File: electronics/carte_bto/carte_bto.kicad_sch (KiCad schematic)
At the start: 59 parts, among them J1 DIN41612_02x32_AB, J2 Conn_01x01, J3 Conn_01x01, J4 Conn_01x01, Q17 MMBT2222A, Q19 MMBT2222A, U1 LTC1859IG_PBF, U2 74AHC541, U3 74AHC541, U4 LT6654AIS6-2.5_TRPBF

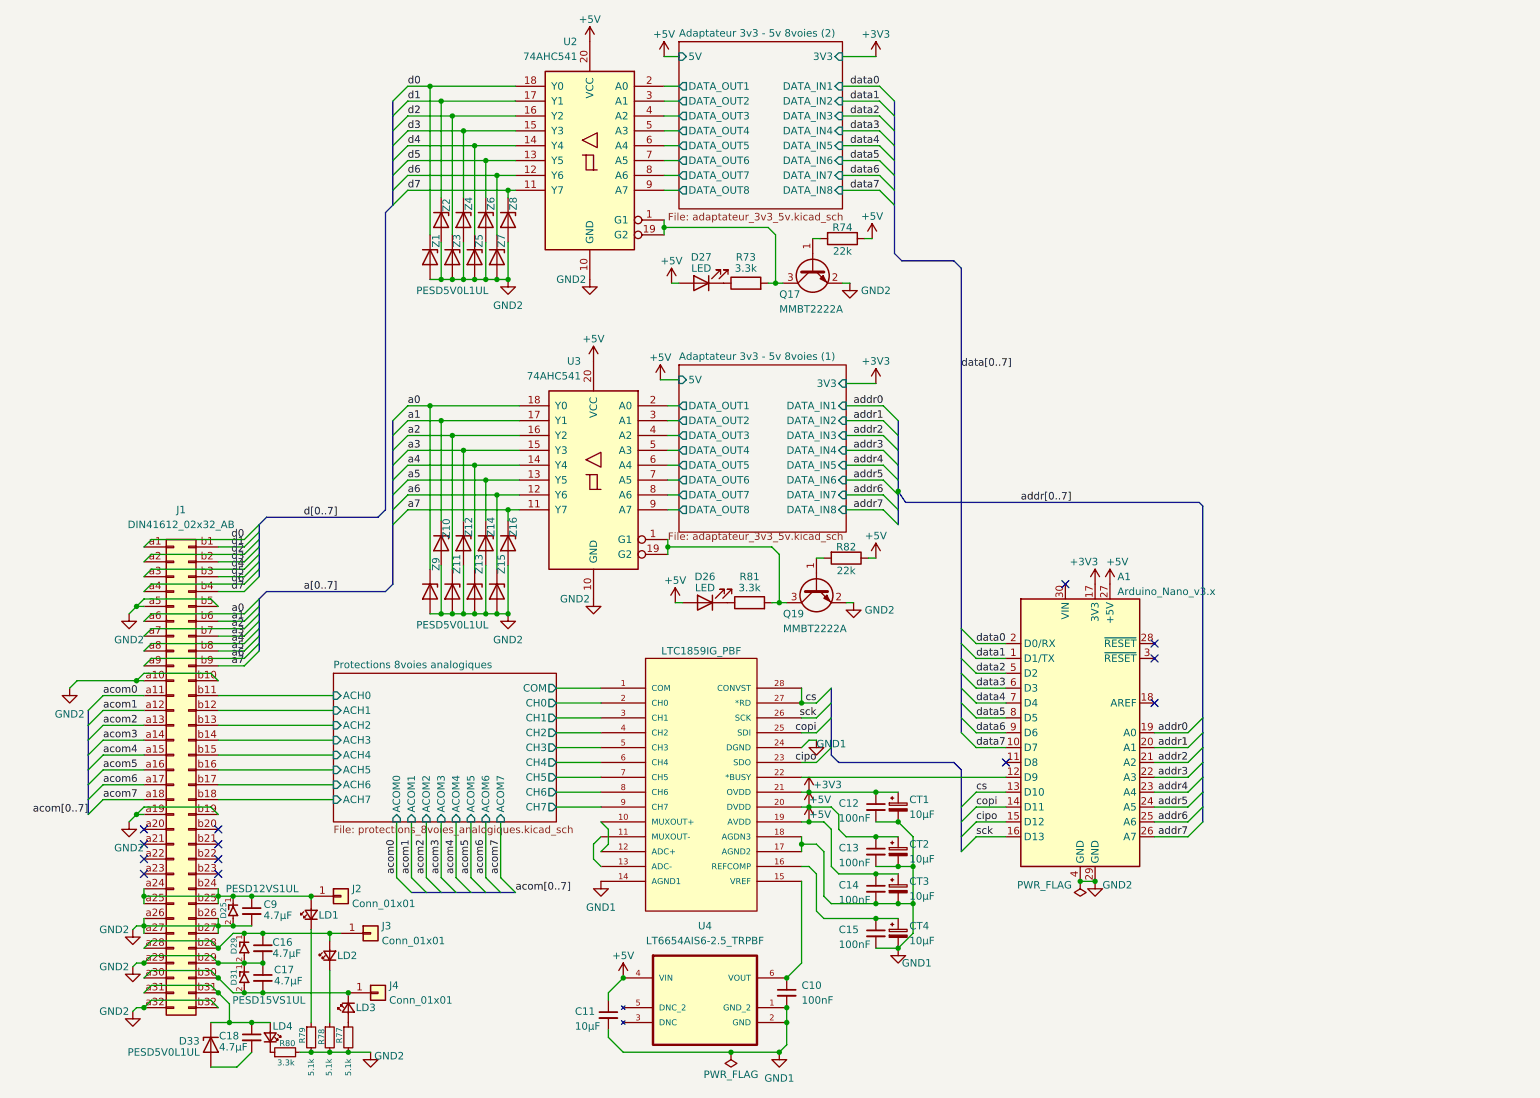
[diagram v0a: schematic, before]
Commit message: BTO schematic: cleanup and documentation
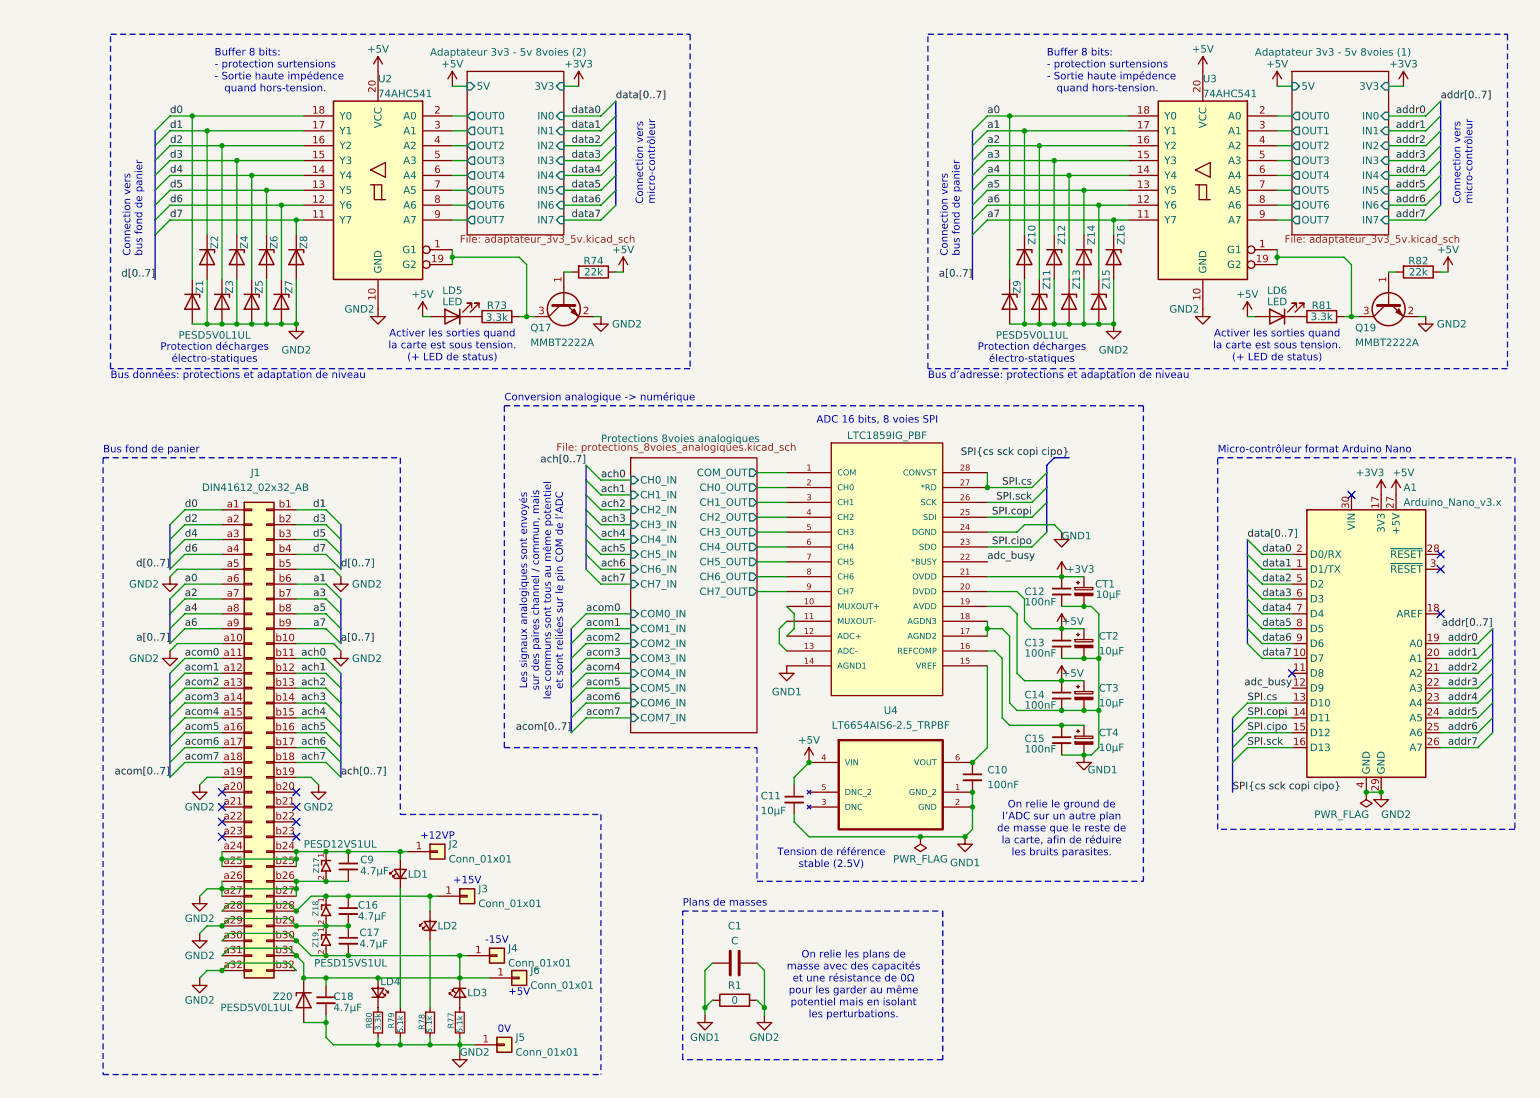
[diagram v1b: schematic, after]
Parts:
- added C1: C, symbol Device:C
- added J5, J6: Conn_01x01, symbol Connector_Generic:Conn_01x01
- added R1: 0, symbol Device:R
- renumbered D27 to LD5, D26 to LD6, D25 to Z17, D29 to Z18, D31 to Z19, D33 to Z20
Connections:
- net GND1: now also C1.1, R1.1
- net GND2: now also C18.2, R80.1, Z20.2 (A), C1.2, J5.1 (Pin_1), R1.2; no longer R80.2
- net at C18.1, J1.a31 (Pin_a31), J1.b31 (Pin_b31)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: now also C17.2, J1.a30 (Pin_a30), J1.b30 (Pin_b30), J4.1 (Pin_1), LD3.1 (K), Z19.2, J6.1 (Pin_1)
- net adc_busy: now reaches A1.12 (D9), U1.22 (*BUSY)
- net at LD4.1 (K): now also R80.2; no longer R80.1
- net Adaptateur 3v3 - 5v 8voies (1)/DATA_OUT1 renamed Adaptateur 3v3 - 5v 8voies (1)/OUT0
- net Adaptateur 3v3 - 5v 8voies (1)/DATA_OUT2 renamed Adaptateur 3v3 - 5v 8voies (1)/OUT1
- net Adaptateur 3v3 - 5v 8voies (1)/DATA_OUT3 renamed Adaptateur 3v3 - 5v 8voies (1)/OUT2
- net Adaptateur 3v3 - 5v 8voies (1)/DATA_OUT4 renamed Adaptateur 3v3 - 5v 8voies (1)/OUT3
- net Adaptateur 3v3 - 5v 8voies (1)/DATA_OUT5 renamed Adaptateur 3v3 - 5v 8voies (1)/OUT4
- net Adaptateur 3v3 - 5v 8voies (1)/DATA_OUT6 renamed Adaptateur 3v3 - 5v 8voies (1)/OUT5
- net Adaptateur 3v3 - 5v 8voies (1)/DATA_OUT7 renamed Adaptateur 3v3 - 5v 8voies (1)/OUT6
- net Adaptateur 3v3 - 5v 8voies (1)/DATA_OUT8 renamed Adaptateur 3v3 - 5v 8voies (1)/OUT7
- net Adaptateur 3v3 - 5v 8voies (2)/DATA_OUT1 renamed Adaptateur 3v3 - 5v 8voies (2)/OUT0
- net Adaptateur 3v3 - 5v 8voies (2)/DATA_OUT2 renamed Adaptateur 3v3 - 5v 8voies (2)/OUT1
- net Adaptateur 3v3 - 5v 8voies (2)/DATA_OUT3 renamed Adaptateur 3v3 - 5v 8voies (2)/OUT2
- net Adaptateur 3v3 - 5v 8voies (2)/DATA_OUT4 renamed Adaptateur 3v3 - 5v 8voies (2)/OUT3
- net Adaptateur 3v3 - 5v 8voies (2)/DATA_OUT5 renamed Adaptateur 3v3 - 5v 8voies (2)/OUT4
- net Adaptateur 3v3 - 5v 8voies (2)/DATA_OUT6 renamed Adaptateur 3v3 - 5v 8voies (2)/OUT5
- net Adaptateur 3v3 - 5v 8voies (2)/DATA_OUT7 renamed Adaptateur 3v3 - 5v 8voies (2)/OUT6
- net Adaptateur 3v3 - 5v 8voies (2)/DATA_OUT8 renamed Adaptateur 3v3 - 5v 8voies (2)/OUT7
- net Protections 8voies analogiques/ACH0 renamed ach0
- net Protections 8voies analogiques/ACH1 renamed ach1
- net Protections 8voies analogiques/ACH2 renamed ach2
- net Protections 8voies analogiques/ACH3 renamed ach3
- net Protections 8voies analogiques/ACH4 renamed ach4
- net Protections 8voies analogiques/ACH5 renamed ach5
- net Protections 8voies analogiques/ACH6 renamed ach6
- net Protections 8voies analogiques/ACH7 renamed ach7
- net Protections 8voies analogiques/CH0 renamed Protections 8voies analogiques/CH0_OUT
- net Protections 8voies analogiques/CH1 renamed Protections 8voies analogiques/CH1_OUT
- net Protections 8voies analogiques/CH2 renamed Protections 8voies analogiques/CH2_OUT
- net Protections 8voies analogiques/CH3 renamed Protections 8voies analogiques/CH3_OUT
- net Protections 8voies analogiques/CH4 renamed Protections 8voies analogiques/CH4_OUT
- net Protections 8voies analogiques/CH5 renamed Protections 8voies analogiques/CH5_OUT
- net Protections 8voies analogiques/CH6 renamed Protections 8voies analogiques/CH6_OUT
- net Protections 8voies analogiques/CH7 renamed Protections 8voies analogiques/CH7_OUT
- net Protections 8voies analogiques/COM renamed Protections 8voies analogiques/COM_OUT
- net cipo renamed SPI.cipo
- net copi renamed SPI.copi
- net cs renamed SPI.cs
- net sck renamed SPI.sck
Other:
- sheet Adaptateur 3v3 - 5v 8voies (1) ports: added IN0, IN1, IN2, IN3, IN4, IN5, IN6, IN7, OUT0, OUT1, OUT2, OUT3, OUT4, OUT5, OUT6, OUT7; removed DATA_IN1, DATA_IN2, DATA_IN3, DATA_IN4, DATA_IN5, DATA_IN6, DATA_IN7, DATA_IN8, DATA_OUT1, DATA_OUT2, DATA_OUT3, DATA_OUT4, DATA_OUT5, DATA_OUT6, DATA_OUT7, DATA_OUT8
- sheet Adaptateur 3v3 - 5v 8voies (2) ports: added IN0, IN1, IN2, IN3, IN4, IN5, IN6, IN7, OUT0, OUT1, OUT2, OUT3, OUT4, OUT5, OUT6, OUT7; removed DATA_IN1, DATA_IN2, DATA_IN3, DATA_IN4, DATA_IN5, DATA_IN6, DATA_IN7, DATA_IN8, DATA_OUT1, DATA_OUT2, DATA_OUT3, DATA_OUT4, DATA_OUT5, DATA_OUT6, DATA_OUT7, DATA_OUT8
- sheet Protections 8voies analogiques ports: added CH0_IN, CH0_OUT, CH1_IN, CH1_OUT, CH2_IN, CH2_OUT, CH3_IN, CH3_OUT, CH4_IN, CH4_OUT, CH5_IN, CH5_OUT, CH6_IN, CH6_OUT, CH7_IN, CH7_OUT, COM0_IN, COM1_IN, COM2_IN, COM3_IN, COM4_IN, COM5_IN, COM6_IN, COM7_IN, COM_OUT; removed ACH0, ACH1, ACH2, ACH3, ACH4, ACH5, ACH6, ACH7, ACOM0, ACOM1, ACOM2, ACOM3, ACOM4, ACOM5, ACOM6, ACOM7, CH0, CH1, CH2, CH3, CH4, CH5, CH6, CH7, COM
- note added: "+12VP"
- note added: "+15V"
- note added: "+5V"
- note added: "-15V"
- note added: "0V"
- note added: "ADC 16 bits, 8 voies SPI"
- note added: "Activer les sorties quand la carte est sous tension. (+ LED de status)"
- note added: "Buffer 8 bits: - protection surtensions - Sortie haute impédence quand hors-tension."
- note added: "Bus données: protections et adaptation de niveau"
- note added: "Bus d’adresse: protections et adaptation de niveau"
- note added: "Bus fond de panier"
- note added: "Connection vers bus fond de panier"
- note added: "Connection vers micro-contrôleur"
- note added: "Conversion analogique -> numérique"
- note added: "Les signaux analogiques sont envoyés sur des paires channel / commun, mais les communs sont tous au même potentiel et sont reliées sur le pin COM de l’ADC"
- note added: "Micro-contrôleur format Arduino Nano"
- note added: "On relie le ground de l’ADC sur un autre plan de masse que le reste de la carte, afin de réduire les bruits parasites."
- note added: "On relie les plans de masse avec des capacités et une résistance de 0Ω pour les garder au même potentiel mais en isolant les perturbations."
- note added: "Plans de masses"
- note added: "Protection décharges électro-statiques"
- note added: "Tension de référence stable (2.5V)"
- moved on the sheet: A1, C10, C11, C12, C13, C14, C15, C16, C17, C18, C9, CT1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

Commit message: BTO: minor schematic fixes & PCB routing.
backup

BTO: Minor fixes on schematic & PCB routing.
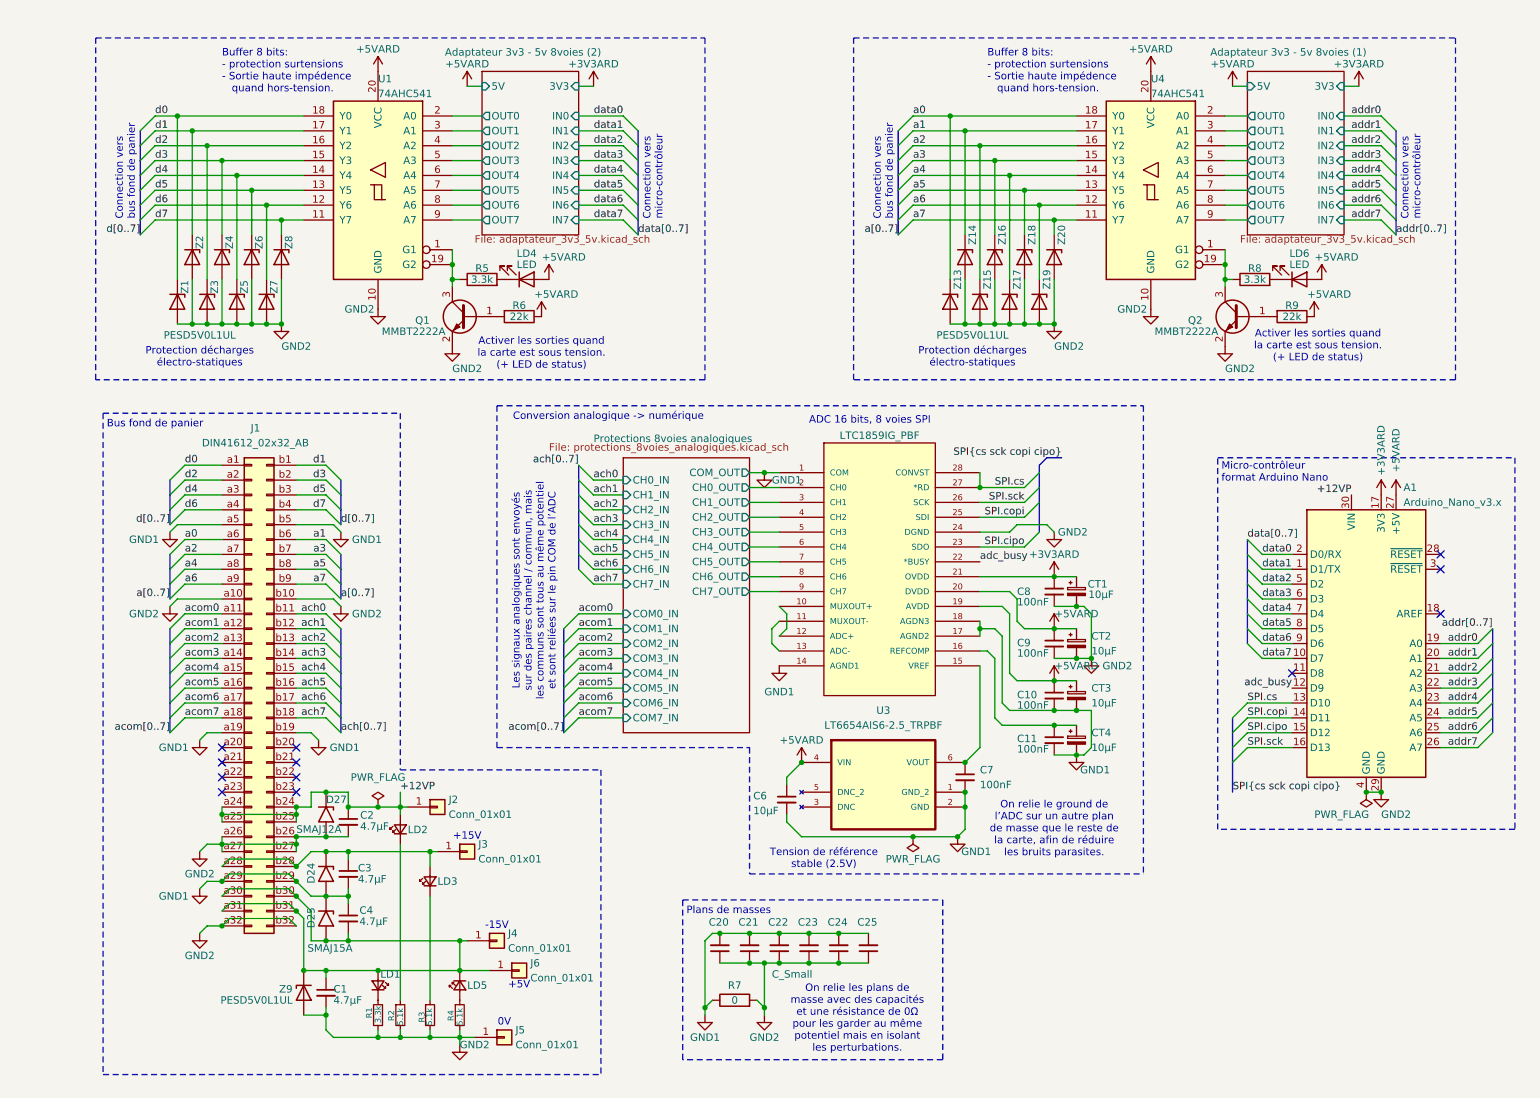
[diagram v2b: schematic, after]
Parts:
- removed C1: C, symbol Device:C
- removed LD5: LED, symbol Device:LED
- removed Q17, Q19: MMBT2222A, Package_TO_SOT_SMD:SOT-23, symbol Transistor_BJT:MMBT2222A
- removed R73, R81: 3.3k, symbol Device:R
- removed R74, R82: 22k, symbol Device:R
- removed U2, U3: 74AHC541, symbol 74xx:74AHC541
- removed Z10, Z11, Z12, Z9: PESD5V0L1UL, Diode_SMD:D_SOD-882, symbol Diode:PESD5V0L1UL
- removed Z17: PESD12VS1UL, PESD12VS1UL:SOD882_T_, symbol PESD12VS1UL:PESD12VS1UL
- removed Z18, Z19: PESD15VS1UL, PESD12VS1UL:SOD882_T_, symbol PESD12VS1UL:PESD15VS1UL
- added C20, C21, C22, C23, C24, C25: C_Small, Capacitor_SMD:C_0805_2012Metric, symbol Device:C_Small
- added D24, D25: SMAJ15A, Diode_SMD:D_SOD-323_HandSoldering, symbol Diode:SMAJ15A
- added D27: SMAJ12A, Diode_SMD:D_SOD-323_HandSoldering, symbol Diode:SMAJ12A
- added LD4: LED, LED_SMD:LED_0805_2012Metric, symbol Device:LED
- added Q1, Q2: MMBT2222A, Package_TO_SOT_SMD:SOT-23, symbol Transistor_BJT:MMBT2222A
- added R5, R8: 3.3k, Resistor_SMD:R_0805_2012Metric, symbol Device:R
- added R6, R9: 22k, Resistor_SMD:R_0805_2012Metric, symbol Device:R
- added U1, U4: 74AHC541, Package_SO:TSSOP-20_4.4x5mm_P0.4mm, symbol 74xx:74AHC541
- added Z17, Z18, Z19, Z20: PESD5V0L1UL, Diode_SMD:D_SOD-882, symbol Diode:PESD5V0L1UL
- C1: renamed from C18; footprint (none) -> Capacitor_SMD:C_0805_2012Metric
- C10: renamed from C14; footprint (none) -> Capacitor_SMD:C_0805_2012Metric
- C11: renamed from C15; footprint (none) -> Capacitor_SMD:C_0805_2012Metric
- C2: renamed from C9; footprint (none) -> Capacitor_SMD:C_0805_2012Metric
- C3: renamed from C16; footprint (none) -> Capacitor_SMD:C_0805_2012Metric
- C4: renamed from C17; footprint (none) -> Capacitor_SMD:C_0805_2012Metric
- C6: renamed from C11; footprint (none) -> Capacitor_SMD:C_0805_2012Metric
- C7: renamed from C10; footprint (none) -> Capacitor_SMD:C_0805_2012Metric
- C8: renamed from C12; footprint (none) -> Capacitor_SMD:C_0805_2012Metric
- C9: renamed from C13; footprint (none) -> Capacitor_SMD:C_0805_2012Metric
- CT1, CT2, CT3, CT4: footprint (none) -> Capacitor_Tantalum_SMD:CP_EIA-2012-12_Kemet-R
- J1: footprint (none) -> Connector_DIN:DIN41612_B_2x32_Male_Horizontal_THT
- J2, J3, J4, J5, J6: footprint (none) -> Connector:Banana_Cliff_FCR7350B_S16N-PC_Horizontal
- LD1: renamed from LD4; footprint (none) -> LED_SMD:LED_0805_2012Metric
- LD2: renamed from LD1; footprint (none) -> LED_SMD:LED_0805_2012Metric
- LD3: renamed from LD2; footprint (none) -> LED_SMD:LED_0805_2012Metric
- LD5: renamed from LD3; footprint (none) -> LED_SMD:LED_0805_2012Metric
- LD6: footprint (none) -> LED_SMD:LED_0805_2012Metric
- R1: renamed from R80; footprint (none) -> Resistor_SMD:R_0805_2012Metric
- R2: renamed from R79; footprint (none) -> Resistor_SMD:R_0805_2012Metric
- R3: renamed from R78; footprint (none) -> Resistor_SMD:R_0805_2012Metric
- R4: renamed from R77; footprint (none) -> Resistor_SMD:R_0805_2012Metric
- R7: renamed from R1; footprint (none) -> Resistor_SMD:R_0805_2012Metric
- U2: renamed from U1; footprint LTC1859IG_PBF:SSOP-28_G -> imported_components:SSOP-28_G
- U3: renamed from U4; footprint LT6654AIS6-2.5_TRPBF:SOT95P280X100-6N -> imported_components:SOT95P280X100-6N
- renumbered Z20 to Z9
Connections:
- net Protections 8voies analogiques/COM_OUT is gone; now on net GND1: U2.1 (COM)
- net Adaptateur 3v3 - 5v 8voies (1)/OUT0: now also U4.2 (A0)
- net Adaptateur 3v3 - 5v 8voies (1)/OUT1: now also U4.3 (A1)
- net Adaptateur 3v3 - 5v 8voies (1)/OUT2: now also U4.4 (A2)
- net Adaptateur 3v3 - 5v 8voies (1)/OUT3: now also U4.5 (A3)
- net Adaptateur 3v3 - 5v 8voies (1)/OUT4: now also U4.6 (A4)
- net Adaptateur 3v3 - 5v 8voies (1)/OUT5: now also U4.7 (A5)
- net Adaptateur 3v3 - 5v 8voies (1)/OUT6: now also U4.8 (A6)
- net Adaptateur 3v3 - 5v 8voies (1)/OUT7: now also U4.9 (A7)
- net Adaptateur 3v3 - 5v 8voies (2)/OUT0: now also U1.2 (A0)
- net Adaptateur 3v3 - 5v 8voies (2)/OUT1: now also U1.3 (A1)
- net Adaptateur 3v3 - 5v 8voies (2)/OUT2: now also U1.4 (A2)
- net Adaptateur 3v3 - 5v 8voies (2)/OUT3: now also U1.5 (A3)
- net Adaptateur 3v3 - 5v 8voies (2)/OUT4: now also U1.6 (A4)
- net Adaptateur 3v3 - 5v 8voies (2)/OUT5: now also U1.7 (A5)
- net Adaptateur 3v3 - 5v 8voies (2)/OUT6: now also U1.8 (A6)
- net Adaptateur 3v3 - 5v 8voies (2)/OUT7: now also U1.9 (A7)
- net GND1: now also C3.2, C4.1, J1.a19 (Pin_a19), J1.a29 (Pin_a29), J1.a5 (Pin_a5), J1.b19 (Pin_b19), J1.b29 (Pin_b29), J1.b5 (Pin_b5), C20.2, C21.2, C22.2, C23.2, C24.2, C25.2, D24.2 (A2), D25.1 (A1); no longer C8.2, C9.2, CT1.2, CT2.2, U2.24 (DGND)
- net GND2: now also C8.2, C9.2, CT1.2, CT2.2, U2.24 (DGND), C20.1, C21.1, C22.1, C23.1, C24.1, C25.1, D27.2 (A2), Q1.2 (E), Q2.2 (E), U1.10 (GND), U4.10 (GND), Z17.2 (A), Z18.2 (A), Z19.2 (A), Z20.2 (A); no longer C3.2, C4.1, J1.a19 (Pin_a19), J1.a29 (Pin_a29), J1.a5 (Pin_a5), J1.b19 (Pin_b19), J1.b29 (Pin_b29), J1.b5 (Pin_b5)
- net a0: now also Z13.1 (K), U4.18 (Y0)
- net a1: now also Z14.1 (K), U4.17 (Y1)
- net a2: now also Z15.1 (K), U4.16 (Y2)
- net a3: now also Z16.1 (K), U4.15 (Y3)
- net a4: now also U4.14 (Y4), Z17.1 (K); no longer Z13.1 (K)
- net a5: now also U4.13 (Y5), Z18.1 (K); no longer Z14.1 (K)
- net a6: now also U4.12 (Y6), Z19.1 (K); no longer Z15.1 (K)
- net a7: now also U4.11 (Y7), Z20.1 (K); no longer Z16.1 (K)
- net d0: now also U1.18 (Y0)
- net d1: now also U1.17 (Y1)
- net d2: now also U1.16 (Y2)
- net d3: now also U1.15 (Y3)
- net d4: now also U1.14 (Y4)
- net d5: now also U1.13 (Y5)
- net d6: now also U1.12 (Y6)
- net d7: now also U1.11 (Y7)
- net at C1.1, C4.2, J1.a30 (Pin_a30)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: now also D25.2 (A2)
- net at LD6.1 (K): now also R8.2
- net at C3.1, J1.a28 (Pin_a28), J1.b28 (Pin_b28)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: now also D24.1 (A1)
- net +12VP: now reaches C2.1, J1.a24 (Pin_a24), J1.a25 (Pin_a25), J1.b24 (Pin_b24), J1.b25 (Pin_b25), J2.1 (Pin_1), LD2.2 (A)
- net +12VP: now also A1.30 (VIN), D27.1 (A1)
- net +3V3 renamed +3V3ARD
- net +5V renamed +5VARD
- net +5VARD: now also LD4.2 (A), R6.1, R9.1, U1.20 (VCC), U4.20 (VCC)
- new net: LD4.1 (K), R5.2
- new net: Q2.3 (C), R8.1, U4.1 (G1), U4.19 (G2)
- new net: Q2.1 (B), R9.2
- new net: Q1.1 (B), R6.2
- new net: Q1.3 (C), R5.1, U1.1 (G1), U1.19 (G2)
- no-connect marks 13 -> 12
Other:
- note removed: "+12VP"
- note removed: "Bus données: protections et adaptation de niveau"
- note removed: "Bus d’adresse: protections et adaptation de niveau"
- moved on the sheet: C1, C10, C11, C2, C3, C4, C6, C7, C8, C9, CT1, CT2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
